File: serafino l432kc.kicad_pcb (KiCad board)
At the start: 4 copper layers, 17.8 x 35.6 mm, 34 parts, among them J1 USB_B_Micro, J2 Conn_01x14, J3 Conn_01x14, Q1 SI3401A-TP, SW1 SW_Push, SW2 SW_Push, U1 AP2112K-3.3, U2 USBLC6-2SC6, U3 STM32L432KCUx, Y1 32.768K

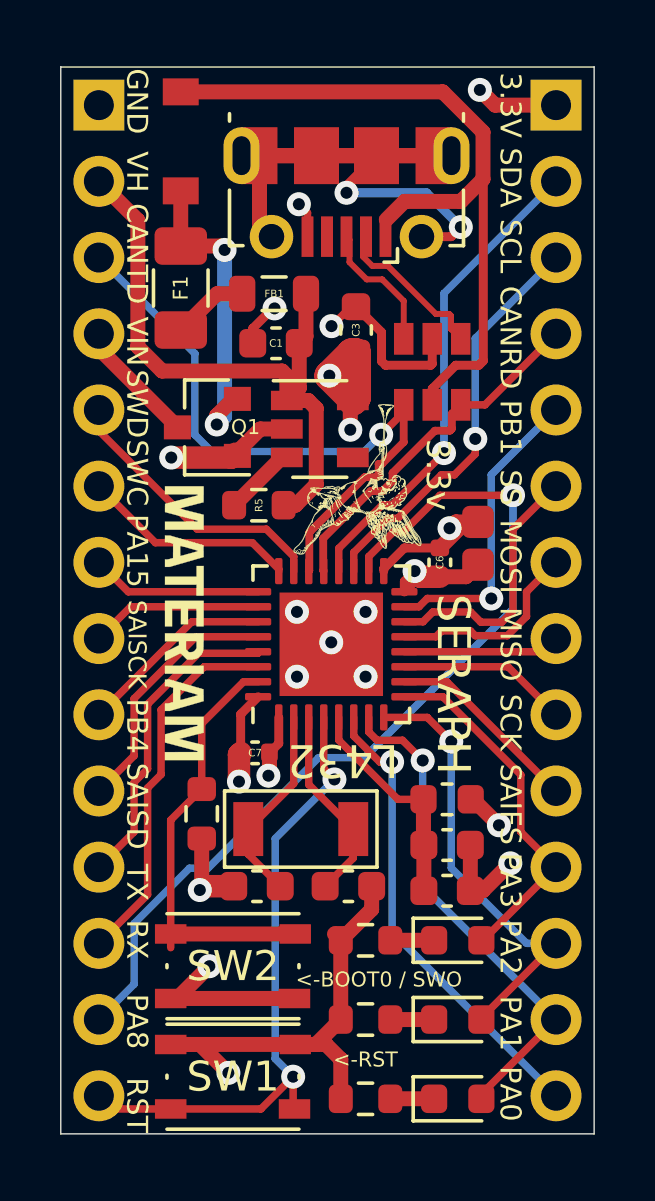
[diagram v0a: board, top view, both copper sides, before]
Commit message: Seraph L4 v1.0
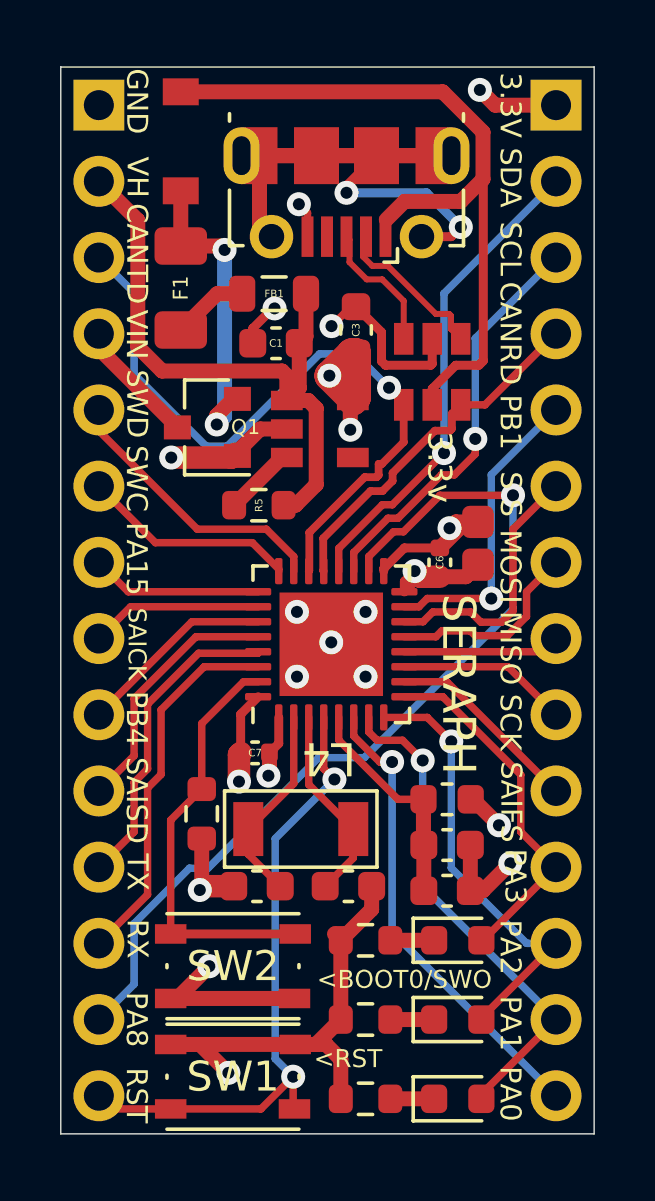
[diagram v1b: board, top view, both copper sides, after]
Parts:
- removed G***: LOGO, serafino l432kc:big_cupid
- removed G***: LOGO, serafino l432kc:cupid
- removed G***: LOGO, serafino l432kc:logo_materiam
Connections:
- net LED0 renamed PA1
- net LED1 renamed PA2
- net LED2 renamed PA3
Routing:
- net CAN_TD: track 22.4 -> 23.8 mm
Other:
- board text added: "* STM32L432KC Ultra Low Power * ARM Cortex M4 @ 80Mhz * 64KB SRAM/256KB Flash * Max Supply VIN: 6.0v/Iout: 600ma * Source/Sink per pin <= 20ma all pins <= 100ma Press RESET while holding BOOT0 to enter DFU programming mode."
- board text added: "<BOOT0/SWO"
- board text added: "<RST"
- board text added: "L4"
- board text added: "S S"
- board text added: "SAICK"
- board text removed: "* STM32L432KC ARM Cortex M4 * 64KB SRAM/256KB Flash/80Mhz * Max Supply Voltage Vin: 6.0v * Power Supply Max Iout: 600ma * Source/Sink per pin <= 20ma * Source/Sink all pins <= 100ma Press RESET while holding BOOT0 to enter DFU mode."
- board text removed: "<-BOOT0 / SWO"
- board text removed: "<-RST"
- board text removed: "L432"
- board text removed: "SAISCK"
- board text removed: "SS"
